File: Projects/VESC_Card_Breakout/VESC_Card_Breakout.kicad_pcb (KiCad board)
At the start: 2 copper layers, 9 parts, among them P1 USB_OTG, P2 CONN_01X02, P3 CONN_01X04, P4 EC90_Flat, P5 CONN_01X02, P6 AMP17614426-2_EDGE, P7 CONN_01X06

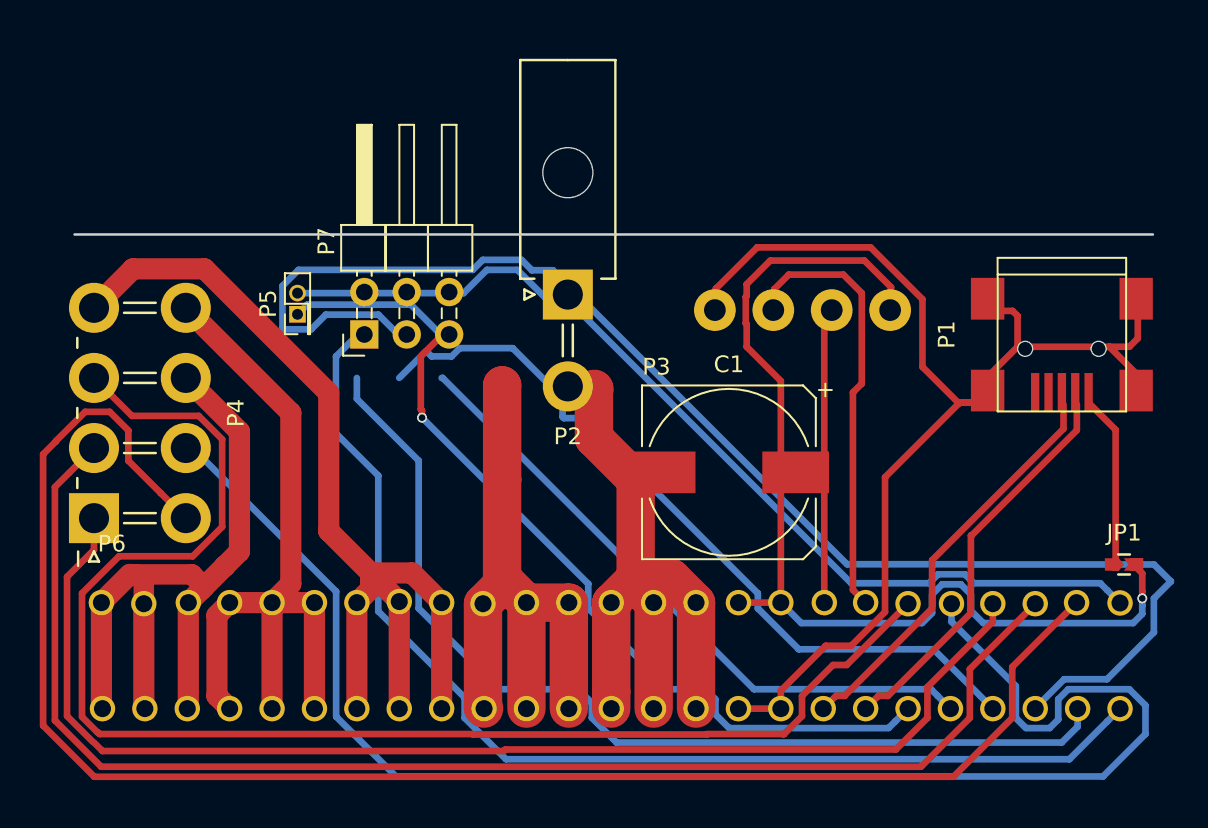
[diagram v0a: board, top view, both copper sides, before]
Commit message: Outline lines added in. PCB finished :D
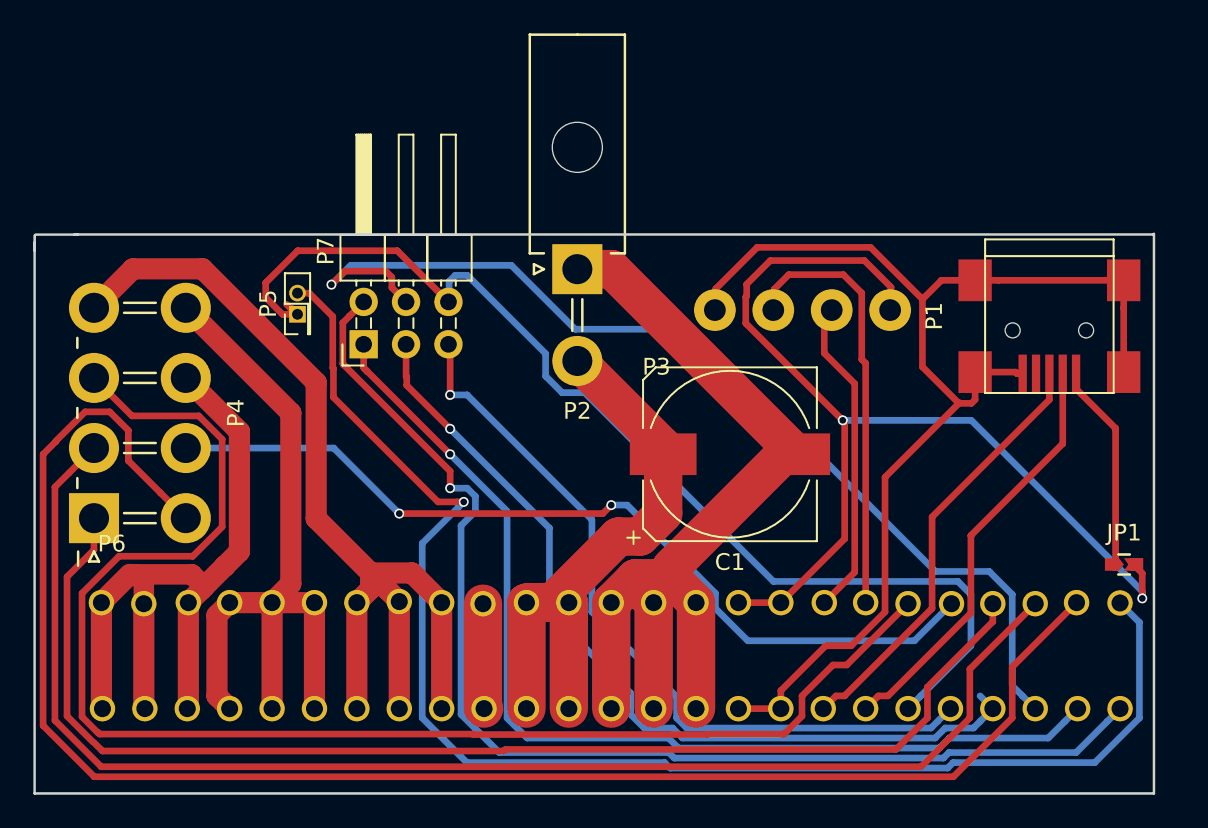
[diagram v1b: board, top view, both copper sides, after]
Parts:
- moved P2 1.63 mm to (160.0, 40.7)
- moved P1 1.33 mm to (188.3, 44.2)
- moved C1 1.09 mm to (169.2, 51.8), turned to 0 degrees
- moved P7 0.59 mm to (147.2, 45.2)
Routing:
- net Net-(P4-Pad6): track 91.3 -> 52.5 mm, vias 0 -> 2
- net Net-(P5-Pad2): track 58.6 -> 84.7 mm, vias 0 -> 1
- net Net-(P6-Pad18): track 84.8 -> 62.8 mm, vias 0 -> 1
- net /Motor_Controller/PGND: track 39.6 -> 56.0 mm
- net /Motor_Controller/GND_AUX: track 53.8 -> 66.3 mm, vias 1 -> 0
- net Net-(P6-Pad20): track 39.2 -> 45.9 mm, vias 0 -> 1
- net /Motor_Controller/VBAT: track 37.2 -> 43.2 mm
- net Net-(P6-Pad19): track 46.7 -> 51.8 mm, vias 0 -> 1
- net Net-(P6-Pad16): track 68.2 -> 71.3 mm, vias 0 -> 1
- net Net-(JP1-Pad1): track 10.4 -> 12.6 mm
- net Net-(P6-Pad17): track 60.1 -> 62.1 mm, vias 0 -> 1
- net /Motor_Controller/CANH/TX: track 18.2 -> 19.7 mm
- net /Motor_Controller/USBDM: track 23.8 -> 25.3 mm
- net /Motor_Controller/USBDP: track 24.5 -> 26.0 mm
- net /GNDD: track 77.0 -> 76.1 mm
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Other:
- board outline added: 67.1 x 33.5 mm
